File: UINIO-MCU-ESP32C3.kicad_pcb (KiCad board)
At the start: 2 copper layers, 60.3 x 20.4 mm, 50 parts, among them J1 Conn_01x15_Male, J2 外接串行下载接口, J3 Conn_01x15_Male, SW1 复位按键, SW2 下载按键, U1 ME6211C33M5G-N, U2 W25Q128JVSSIQ, U3 ESP32-C3, U4 CH343P, Y1 40MHz

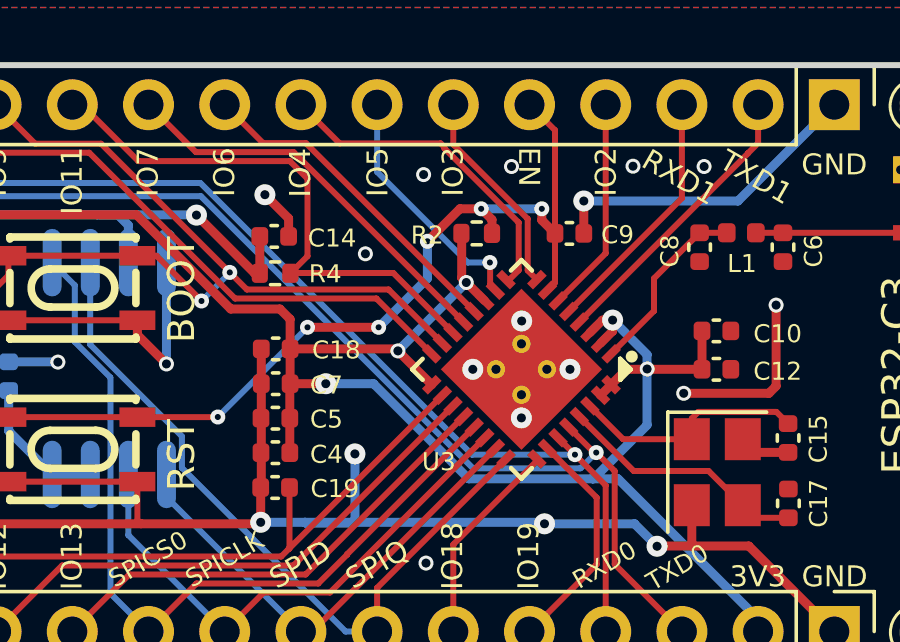
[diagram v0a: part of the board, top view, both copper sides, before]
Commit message: Complete wiring.
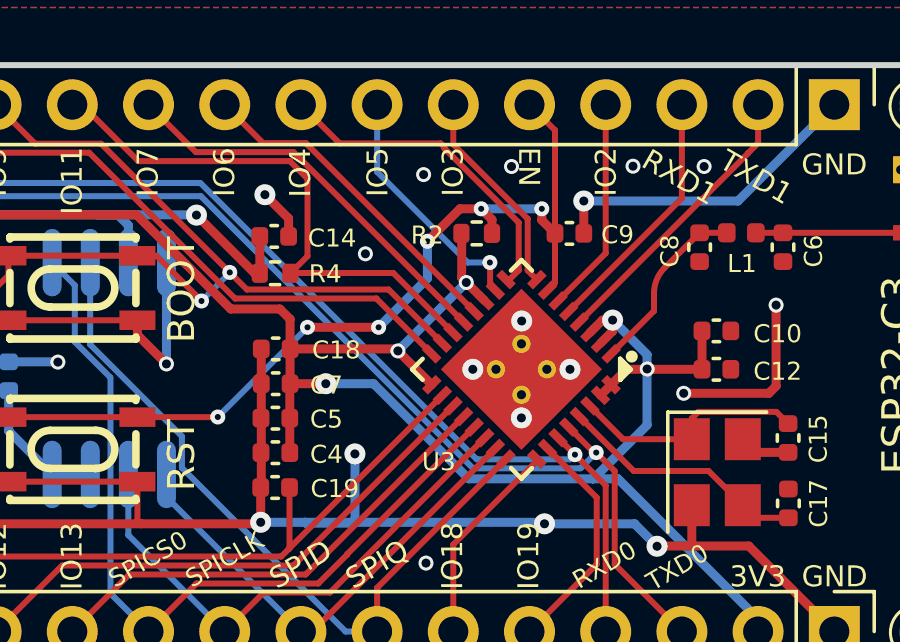
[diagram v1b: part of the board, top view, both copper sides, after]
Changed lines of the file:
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@@
   (segment (start 134.37 111.72) (end 138.18 111.72) (width 0.5) (layer "B.Cu") (net 4))
   (segment (start 129.62 100.52) (end 129.62 106.97) (width 0.5) (layer "B.Cu") (net 4))
-  (segment (start 167.73 101.035903) (end 167.73 99.95) (width 0.2) (layer "F.Cu") (net 5))
   (segment (start 170.155 98.43) (end 169.25 98.43) (width 0.2) (layer "F.Cu") (net 5))
+  (segment (start 168.083553 99.596446) (end 169.25 98.43) (width 0.2) (layer "F.Cu") (net 5))
+  (segment (start 167.73 100.45) (end 167.73 101.035903) (width 0.2) (layer "F.Cu") (net 5))
   (segment (start 166.300677 102.465226) (end 167.73 101.035903) (width 0.2) (layer "F.Cu") (net 5))
-  (segment (start 167.73 99.95) (end 169.25 98.43) (width 0.2) (layer "F.Cu") (net 5))
+  (arc (start 167.73 100.45) (mid 167.821884 99.988059) (end 168.083552 99.596445) (width 0.2) (layer "F.Cu") (net 5))
   (segment (start 164.43 98.45) (end 164.43 100.093263) (width 0.2) (layer "F.Cu") (net 6))
   (segment (start 153.185 104.575) (end 150.51 104.575) (width 0.2) (layer "F.Cu") (net 6))
@@
   (via (at 131.62 96.7605) (size 0.5) (drill 0.2) (layers "F.Cu" "B.Cu") (net 23))
   (via (at 131.63 101.73) (size 0.5) (drill 0.2) (layers "F.Cu" "B.Cu") (net 23))
+  (segment (start 165.095185 105.824815) (end 164.94 105.98) (width 0.2) (layer "B.Cu") (net 23))
+  (segment (start 131.63 97.6695) (end 131.62 97.6595) (width 0.2) (layer "B.Cu") (net 23))
+  (segment (start 161.82 105.98) (end 152.61 96.77) (width 0.2) (layer "B.Cu") (net 23))
+  (segment (start 164.94 105.98) (end 161.82 105.98) (width 0.2) (layer "B.Cu") (net 23))
+  (segment (start 131.62 96.77) (end 130.57 95.72) (width 0.2) (layer "B.Cu") (net 23))
   (segment (start 130.57 95.72) (end 130.57 94.15) (width 0.2) (layer "B.Cu") (net 23))
-  (segment (start 131.63 97.6695) (end 131.62 97.6595) (width 0.2) (layer "B.Cu") (net 23))
-  (segment (start 161.664815 105.824815) (end 152.61 96.77) (width 0.2) (layer "B.Cu") (net 23))
   (segment (start 131.63 101.73) (end 131.63 97.6695) (width 0.2) (layer "B.Cu") (net 23))
   (segment (start 152.61 96.77) (end 131.62 96.77) (width 0.2) (layer "B.Cu") (net 23))
-  (segment (start 131.62 96.77) (end 130.57 95.72) (width 0.2) (layer "B.Cu") (net 23))
-  (segment (start 165.095185 105.824815) (end 161.664815 105.824815) (width 0.2) (layer "B.Cu") (net 23))
   (segment (start 130.96 101.13) (end 134.259 101.13) (width 0.2) (layer "F.Cu") (net 24))
   (segment (start 165.804447 105.755553) (end 165.73303 105.755553) (width 0.2) (layer "F.Cu") (net 24))
